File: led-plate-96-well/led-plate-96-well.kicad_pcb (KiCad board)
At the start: 4 copper layers, 175 x 100 mm, 31 parts, among them J1 RAPC722X, U1 A000053, U2 TLC5947RHB

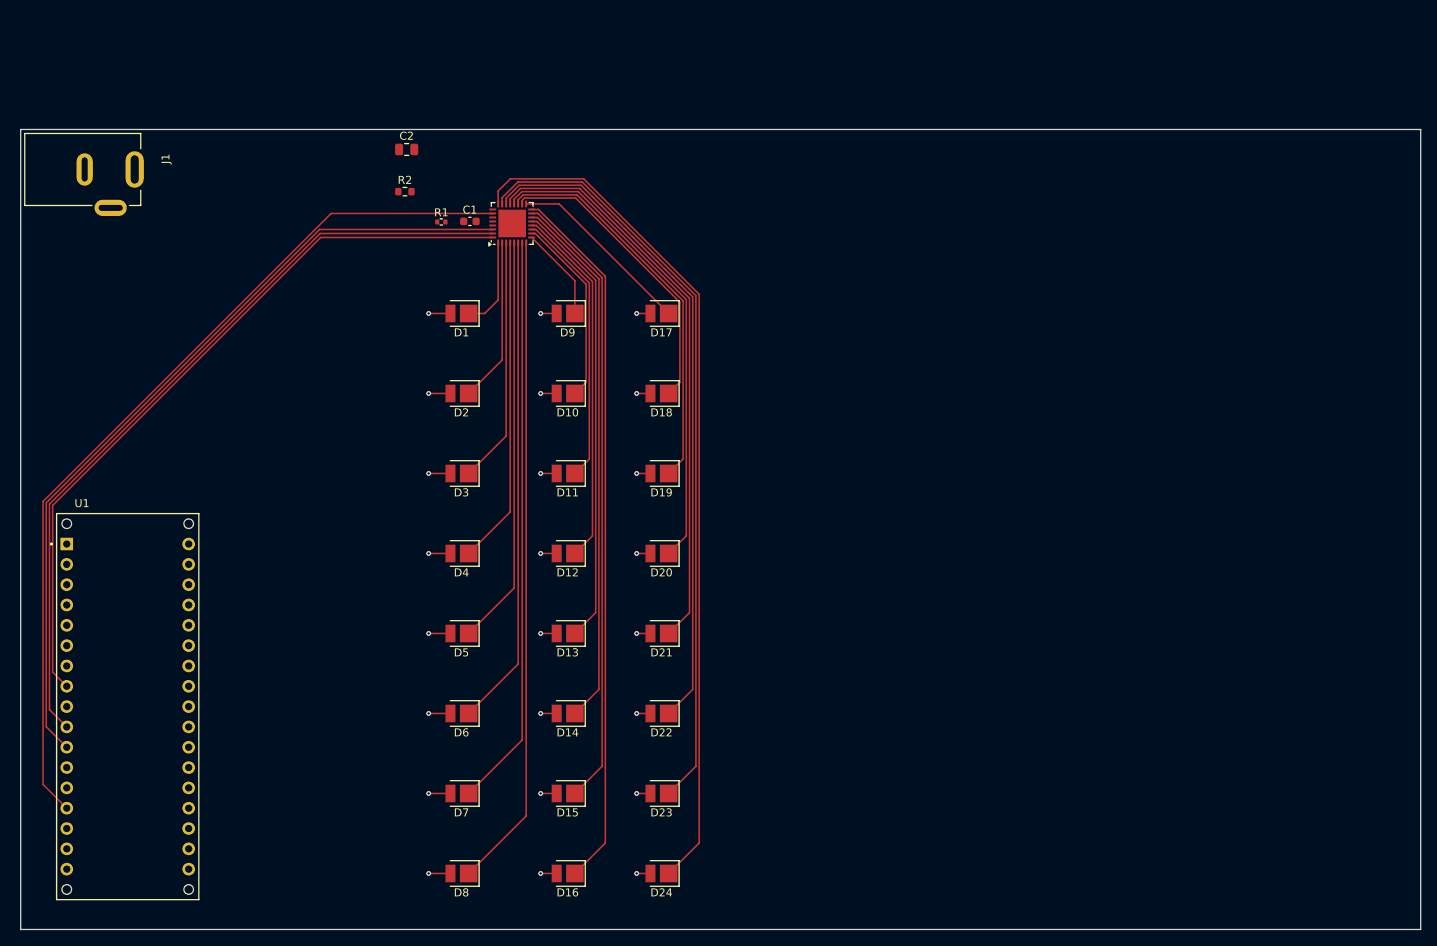
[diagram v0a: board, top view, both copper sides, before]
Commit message: layout leds
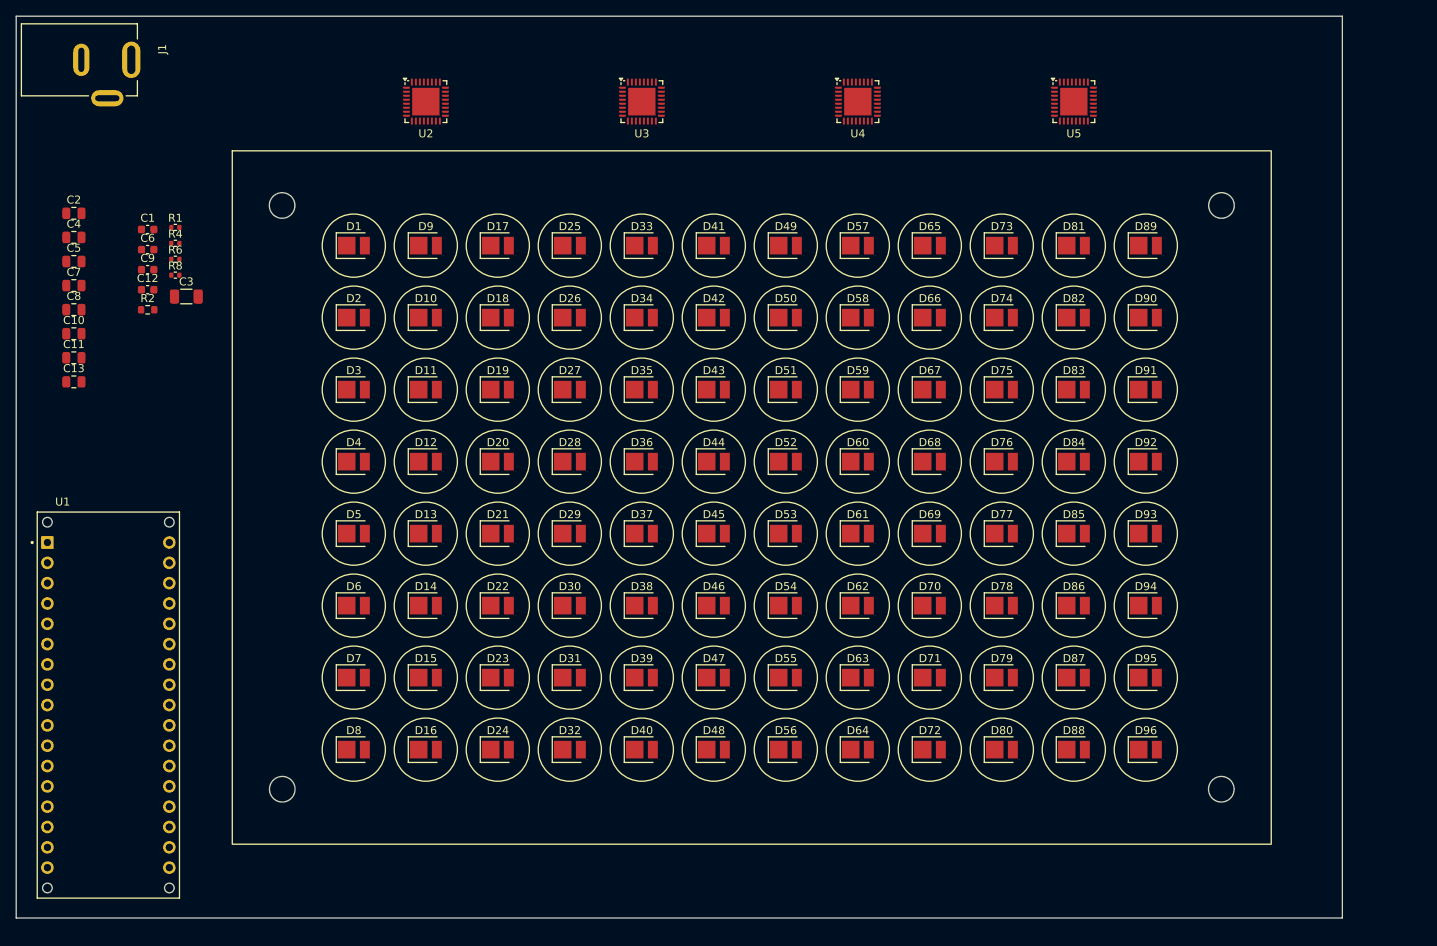
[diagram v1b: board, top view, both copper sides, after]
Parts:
- added C10: 10uF, Capacitor_SMD:C_0805_2012Metric, F.Cu at (50.6, 69.5)
- added C11: 10uF, Capacitor_SMD:C_0805_2012Metric, F.Cu at (50.6, 72.5)
- added C12: 100nF, Capacitor_SMD:C_0603_1608Metric, F.Cu at (59.9, 64.0)
- added C13: 10uF, Capacitor_SMD:C_0805_2012Metric, F.Cu at (50.6, 75.5)
- added C3: 100uF, Capacitor_SMD:C_1206_3216Metric, F.Cu at (64.7, 64.9)
- added C4: 10uF, Capacitor_SMD:C_0805_2012Metric, F.Cu at (50.6, 57.5)
- added C5: 10uF, Capacitor_SMD:C_0805_2012Metric, F.Cu at (50.6, 60.5)
- added C6: 100nF, Capacitor_SMD:C_0603_1608Metric, F.Cu at (59.9, 59.0)
- added C7: 10uF, Capacitor_SMD:C_0805_2012Metric, F.Cu at (50.6, 63.5)
- added C8: 10uF, Capacitor_SMD:C_0805_2012Metric, F.Cu at (50.6, 66.5)
- added C9: 100nF, Capacitor_SMD:C_0603_1608Metric, F.Cu at (59.9, 61.5)
- added D25: LED, SMD2835_WITH_STEP:LED_PLCC_2835, F.Cu at (112.7, 58.5)
- added D26: LED, SMD2835_WITH_STEP:LED_PLCC_2835, F.Cu at (112.7, 67.5)
- added D27: LED, SMD2835_WITH_STEP:LED_PLCC_2835, F.Cu at (112.7, 76.5)
- added D28: LED, SMD2835_WITH_STEP:LED_PLCC_2835, F.Cu at (112.7, 85.5)
- added D29: LED, SMD2835_WITH_STEP:LED_PLCC_2835, F.Cu at (112.7, 94.5)
- added D30: LED, SMD2835_WITH_STEP:LED_PLCC_2835, F.Cu at (112.7, 103.5)
- added D31: LED, SMD2835_WITH_STEP:LED_PLCC_2835, F.Cu at (112.7, 112.5)
- added D32: LED, SMD2835_WITH_STEP:LED_PLCC_2835, F.Cu at (112.7, 121.5)
- added D33: LED, SMD2835_WITH_STEP:LED_PLCC_2835, F.Cu at (121.7, 58.5)
- added D34: LED, SMD2835_WITH_STEP:LED_PLCC_2835, F.Cu at (121.7, 67.5)
- added D35: LED, SMD2835_WITH_STEP:LED_PLCC_2835, F.Cu at (121.7, 76.5)
- added D36: LED, SMD2835_WITH_STEP:LED_PLCC_2835, F.Cu at (121.7, 85.5)
- added D37: LED, SMD2835_WITH_STEP:LED_PLCC_2835, F.Cu at (121.7, 94.5)
- added D38: LED, SMD2835_WITH_STEP:LED_PLCC_2835, F.Cu at (121.7, 103.5)
- added D39: LED, SMD2835_WITH_STEP:LED_PLCC_2835, F.Cu at (121.7, 112.5)
- added D40: LED, SMD2835_WITH_STEP:LED_PLCC_2835, F.Cu at (121.7, 121.5)
- added D41: LED, SMD2835_WITH_STEP:LED_PLCC_2835, F.Cu at (130.7, 58.5)
- added D42: LED, SMD2835_WITH_STEP:LED_PLCC_2835, F.Cu at (130.7, 67.5)
- added D43: LED, SMD2835_WITH_STEP:LED_PLCC_2835, F.Cu at (130.7, 76.5)
- added D44: LED, SMD2835_WITH_STEP:LED_PLCC_2835, F.Cu at (130.7, 85.5)
- added D45: LED, SMD2835_WITH_STEP:LED_PLCC_2835, F.Cu at (130.7, 94.5)
- added D46: LED, SMD2835_WITH_STEP:LED_PLCC_2835, F.Cu at (130.7, 103.5)
- added D47: LED, SMD2835_WITH_STEP:LED_PLCC_2835, F.Cu at (130.7, 112.5)
- added D48: LED, SMD2835_WITH_STEP:LED_PLCC_2835, F.Cu at (130.7, 121.5)
- added D49: LED, SMD2835_WITH_STEP:LED_PLCC_2835, F.Cu at (139.7, 58.5)
- added D50: LED, SMD2835_WITH_STEP:LED_PLCC_2835, F.Cu at (139.7, 67.5)
- added D51: LED, SMD2835_WITH_STEP:LED_PLCC_2835, F.Cu at (139.7, 76.5)
- added D52: LED, SMD2835_WITH_STEP:LED_PLCC_2835, F.Cu at (139.7, 85.5)
- added D53: LED, SMD2835_WITH_STEP:LED_PLCC_2835, F.Cu at (139.7, 94.5)
- added D54: LED, SMD2835_WITH_STEP:LED_PLCC_2835, F.Cu at (139.7, 103.5)
- added D55: LED, SMD2835_WITH_STEP:LED_PLCC_2835, F.Cu at (139.7, 112.5)
- added D56: LED, SMD2835_WITH_STEP:LED_PLCC_2835, F.Cu at (139.7, 121.5)
- added D57: LED, SMD2835_WITH_STEP:LED_PLCC_2835, F.Cu at (148.7, 58.5)
- added D58: LED, SMD2835_WITH_STEP:LED_PLCC_2835, F.Cu at (148.7, 67.5)
- added D59: LED, SMD2835_WITH_STEP:LED_PLCC_2835, F.Cu at (148.7, 76.5)
- added D60: LED, SMD2835_WITH_STEP:LED_PLCC_2835, F.Cu at (148.7, 85.5)
- added D61: LED, SMD2835_WITH_STEP:LED_PLCC_2835, F.Cu at (148.7, 94.5)
- added D62: LED, SMD2835_WITH_STEP:LED_PLCC_2835, F.Cu at (148.7, 103.5)
- added D63: LED, SMD2835_WITH_STEP:LED_PLCC_2835, F.Cu at (148.7, 112.5)
- added D64: LED, SMD2835_WITH_STEP:LED_PLCC_2835, F.Cu at (148.7, 121.5)
- added D65: LED, SMD2835_WITH_STEP:LED_PLCC_2835, F.Cu at (157.7, 58.5)
- added D66: LED, SMD2835_WITH_STEP:LED_PLCC_2835, F.Cu at (157.7, 67.5)
- added D67: LED, SMD2835_WITH_STEP:LED_PLCC_2835, F.Cu at (157.7, 76.5)
- added D68: LED, SMD2835_WITH_STEP:LED_PLCC_2835, F.Cu at (157.7, 85.5)
- added D69: LED, SMD2835_WITH_STEP:LED_PLCC_2835, F.Cu at (157.7, 94.5)
- added D70: LED, SMD2835_WITH_STEP:LED_PLCC_2835, F.Cu at (157.7, 103.5)
- added D71: LED, SMD2835_WITH_STEP:LED_PLCC_2835, F.Cu at (157.7, 112.5)
- added D72: LED, SMD2835_WITH_STEP:LED_PLCC_2835, F.Cu at (157.7, 121.5)
- added D73: LED, SMD2835_WITH_STEP:LED_PLCC_2835, F.Cu at (166.7, 58.5)
- added D74: LED, SMD2835_WITH_STEP:LED_PLCC_2835, F.Cu at (166.7, 67.5)
- added D75: LED, SMD2835_WITH_STEP:LED_PLCC_2835, F.Cu at (166.7, 76.5)
- added D76: LED, SMD2835_WITH_STEP:LED_PLCC_2835, F.Cu at (166.7, 85.5)
- added D77: LED, SMD2835_WITH_STEP:LED_PLCC_2835, F.Cu at (166.7, 94.5)
- added D78: LED, SMD2835_WITH_STEP:LED_PLCC_2835, F.Cu at (166.7, 103.5)
- added D79: LED, SMD2835_WITH_STEP:LED_PLCC_2835, F.Cu at (166.7, 112.5)
- added D80: LED, SMD2835_WITH_STEP:LED_PLCC_2835, F.Cu at (166.7, 121.5)
- added D81: LED, SMD2835_WITH_STEP:LED_PLCC_2835, F.Cu at (175.7, 58.5)
- added D82: LED, SMD2835_WITH_STEP:LED_PLCC_2835, F.Cu at (175.7, 67.5)
- added D83: LED, SMD2835_WITH_STEP:LED_PLCC_2835, F.Cu at (175.7, 76.5)
- added D84: LED, SMD2835_WITH_STEP:LED_PLCC_2835, F.Cu at (175.7, 85.5)
- added D85: LED, SMD2835_WITH_STEP:LED_PLCC_2835, F.Cu at (175.7, 94.5)
- added D86: LED, SMD2835_WITH_STEP:LED_PLCC_2835, F.Cu at (175.7, 103.5)
- added D87: LED, SMD2835_WITH_STEP:LED_PLCC_2835, F.Cu at (175.7, 112.5)
- added D88: LED, SMD2835_WITH_STEP:LED_PLCC_2835, F.Cu at (175.7, 121.5)
- added D89: LED, SMD2835_WITH_STEP:LED_PLCC_2835, F.Cu at (184.7, 58.5)
- added D90: LED, SMD2835_WITH_STEP:LED_PLCC_2835, F.Cu at (184.7, 67.5)
- added D91: LED, SMD2835_WITH_STEP:LED_PLCC_2835, F.Cu at (184.7, 76.5)
- added D92: LED, SMD2835_WITH_STEP:LED_PLCC_2835, F.Cu at (184.7, 85.5)
- added D93: LED, SMD2835_WITH_STEP:LED_PLCC_2835, F.Cu at (184.7, 94.5)
- added D94: LED, SMD2835_WITH_STEP:LED_PLCC_2835, F.Cu at (184.7, 103.5)
- added D95: LED, SMD2835_WITH_STEP:LED_PLCC_2835, F.Cu at (184.7, 112.5)
- added D96: LED, SMD2835_WITH_STEP:LED_PLCC_2835, F.Cu at (184.7, 121.5)
- added R4: 2.49kΩ, Resistor_SMD:R_0402_1005Metric, F.Cu at (63.3, 58.2)
- added R6: 2.49kΩ, Resistor_SMD:R_0402_1005Metric, F.Cu at (63.3, 60.2)
- added R8: 2.49kΩ, Resistor_SMD:R_0402_1005Metric, F.Cu at (63.3, 62.2)
- added REF**: plate_adapater_96_well, plate_adapater_96_well:plate_adapater_96_well, F.Cu at (135.4, 90.0)
- added U3: TLC5947RHB, Package_DFN_QFN:QFN-32-1EP_5x5mm_P0.5mm_EP3.45x3.45mm, F.Cu at (121.7, 40.5)
- added U4: TLC5947RHB, Package_DFN_QFN:QFN-32-1EP_5x5mm_P0.5mm_EP3.45x3.45mm, F.Cu at (148.7, 40.5)
- added U5: TLC5947RHB, Package_DFN_QFN:QFN-32-1EP_5x5mm_P0.5mm_EP3.45x3.45mm, F.Cu at (175.7, 40.5)
- moved C2 42.4 mm to (50.6, 54.5)
- moved C1 40.3 mm to (59.9, 56.5)
- moved R2 35.4 mm to (59.9, 66.5)
- moved R1 33.3 mm to (63.3, 56.2)
- moved D24 25.6 mm to (103.7, 121.5), turned to 0 degrees
- moved D23 25.1 mm to (103.7, 112.5), turned to 0 degrees
- moved D22 24.5 mm to (103.7, 103.5), turned to 0 degrees
- moved D21 24.0 mm to (103.7, 94.5), turned to 0 degrees
- moved D16 23.5 mm to (94.7, 121.5), turned to 0 degrees
- moved D20 23.5 mm to (103.7, 85.5), turned to 0 degrees
- moved D19 23.0 mm to (103.7, 76.5), turned to 0 degrees
- moved D15 22.9 mm to (94.7, 112.5), turned to 0 degrees
- moved D18 22.5 mm to (103.7, 67.5), turned to 0 degrees
- moved D14 22.3 mm to (94.7, 103.5), turned to 0 degrees
- moved D17 22.1 mm to (103.7, 58.5), turned to 0 degrees
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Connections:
- U1 pad 30: Net-(U1-RESET-Pad30) -> unconnected-(U1-RESET-Pad30)_1
- U1 pad 5: Net-(U1-RESET-Pad30) -> unconnected-(U1-RESET-Pad30)
- U2 pad 25: unconnected-(U2-SOUT-Pad25) -> Net-(U2-SOUT)
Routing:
- net Net-(U1-9(PWM)/A9): track 110.7 -> 0.00 mm
- net Net-(D24-K): track 107.3 -> 0.00 mm
- net Net-(U1-6(PWM)/A7): track 101.6 -> 0.00 mm
- net Net-(U1-5(PWM)): track 98.2 -> 0.00 mm
- net Net-(D23-K): track 95.3 -> 0.00 mm
- net Net-(U1-3(PWM)/SCL): track 92.2 -> 0.00 mm
- net Net-(D16-K): track 88.9 -> 0.00 mm
- net Net-(D22-K): track 83.8 -> 0.00 mm
- net Net-(D8-K): track 81.8 -> 0.00 mm
- net Net-(D15-K): track 78.0 -> 0.00 mm
- net Net-(D21-K): track 72.3 -> 0.00 mm
- net Net-(D7-K): track 71.6 -> 0.00 mm
- net Net-(D14-K): track 67.1 -> 0.00 mm
- net Net-(D6-K): track 61.4 -> 0.00 mm
- net Net-(D20-K): track 60.7 -> 0.00 mm
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- removed copper zone on In2.Cu, net +5V
- removed copper zone on In1.Cu, net GND
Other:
- board size 175 x 100 mm -> 165.8 x 112.7 mm
